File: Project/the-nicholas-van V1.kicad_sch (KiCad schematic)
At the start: 39 parts, among them J1 JST SH, J2 Pico EZmate, J3 USB_C sink board 1.3mm, J4 Conn_01x05, J5 ARGB, SW1 BOOT0, U1 STM32F401CBUx, U2 XC6206PxxxMR, U3 74AHCT1G125, Y1 8 MHz

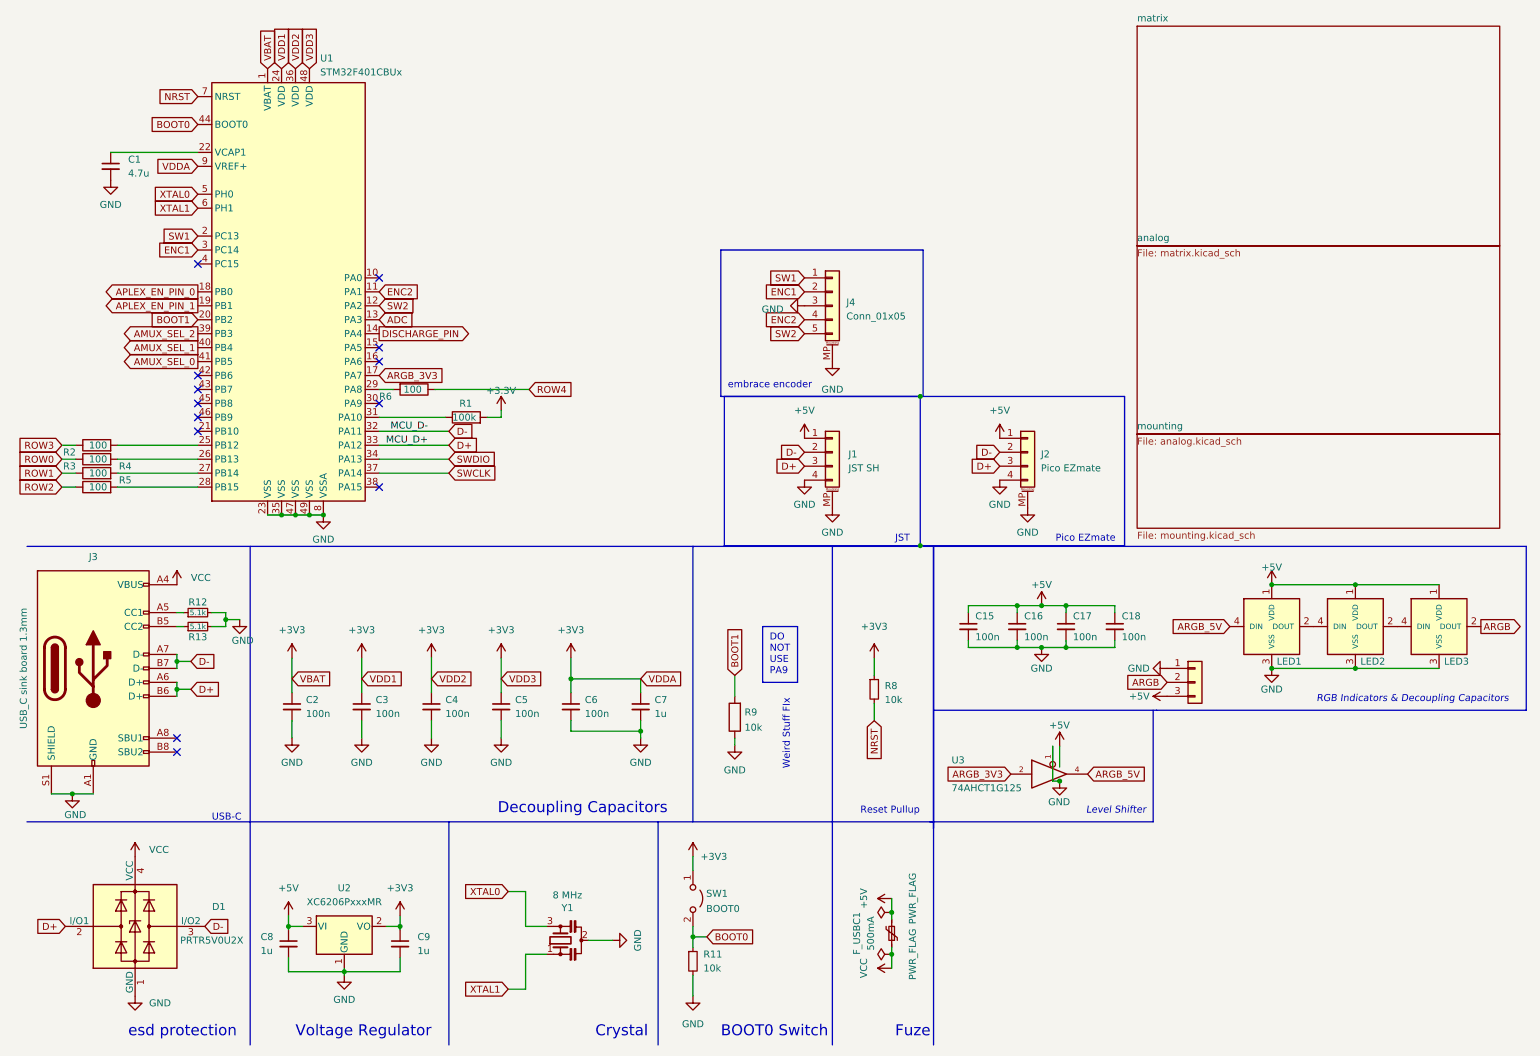
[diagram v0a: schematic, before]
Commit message: update revision
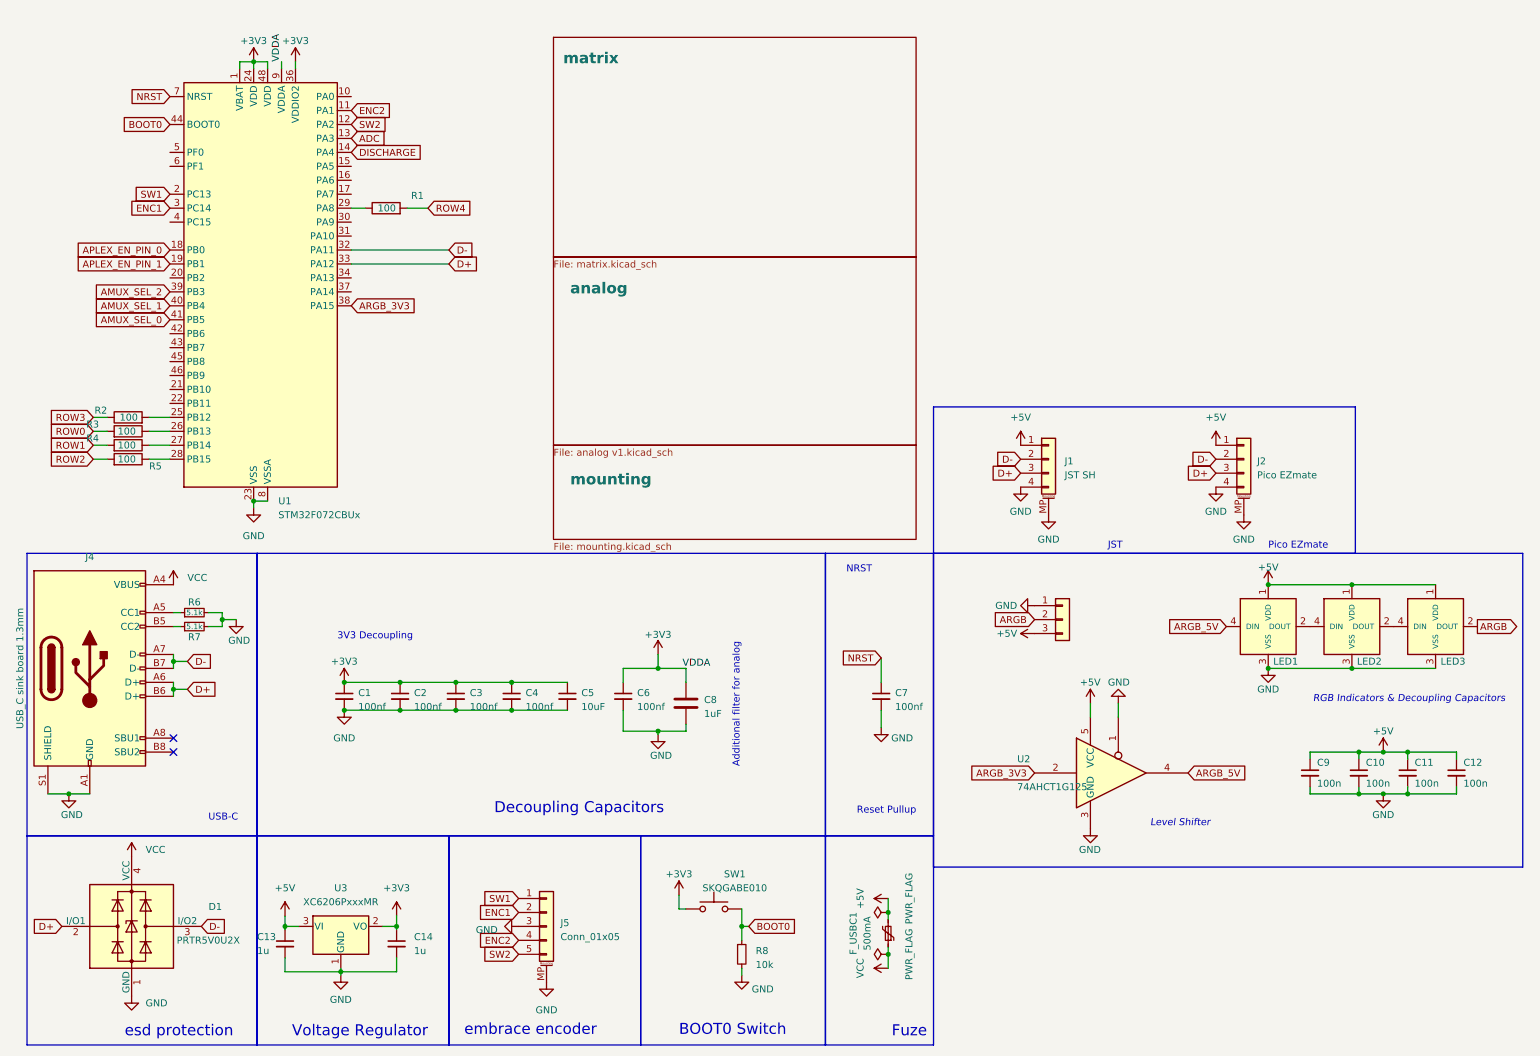
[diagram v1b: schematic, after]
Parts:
- removed R11: 10k, Resistor_SMD:R_0402_1005Metric, symbol Device:R_Small
- removed R6: 100, Resistor_SMD:R_0402_1005Metric, symbol Device:R
- removed R9: 10k, Resistor_SMD:R_0402_1005Metric, symbol Device:R
- removed SW1: BOOT0, Connector_PinHeader_2.54mm:PinHeader_1x02_P2.54mm_Vertical, symbol Jumper:Jumper_2_Open
- removed U1: STM32F401CBUx, Package_DFN_QFN:QFN-48-1EP_7x7mm_P0.5mm_EP5.6x5.6mm, symbol MCU_ST_STM32F4:STM32F401CBUx
- removed Y1: 8 MHz, Crystal:Resonator_SMD_Murata_CSTxExxV-3Pin_3.0x1.1mm, symbol Device:Resonator_Small
- added C8: 1uF, Capacitor_SMD:C_0402_1005Metric, symbol Device:C
- added SW1: SKQGABE010, Connector_PinSocket_2.54mm:PinSocket_1x02_P2.54mm_Vertical, symbol Switch:SW_Push
- added U1: STM32F072CBUx, Package_QFP:LQFP-48_7x7mm_P0.5mm, symbol MCU_ST_STM32F0:STM32F072CBUx
- C1: value 4.7u -> 100nf
- C2, C3, C4, C6: value 100n -> 100nf
- C5: value 100n -> 10uF
- C7: value 1u -> 100nf
- R1: value 100k -> 100; LCSC C25741 -> C25076
- renumbered C16 to C10, C17 to C11, C18 to C12, C8 to C13, C9 to C14, C15 to C9, J5 to J3, J3 to J4, J4 to J5, R12 to R6, R13 to R7, U3 to U2, U2 to U3
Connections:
- net +3V3: now also C1.1, C8.1, SW1.1, U1.1 (VBAT), U1.24 (VDD), U1.36 (VDDIO2), U1.48 (VDD), U1.9 (VDDA); no longer C7.1, R1.2, R8.1
- net ADC: now also U1.13 (PA3)
- net AMUX_SEL_0: now also U1.41 (PB5)
- net AMUX_SEL_1: now also U1.40 (PB4)
- net AMUX_SEL_2: now also U1.39 (PB3)
- net APLEX_EN_PIN_0: now also U1.18 (PB0)
- net APLEX_EN_PIN_1: now also U1.19 (PB1)
- net ARGB_3V3: now also U1.38 (PA15)
- net BOOT0: now also R8.1, SW1.2, U1.44 (BOOT0)
- net D+: now also U1.33 (PA12)
- net D-: now also U1.32 (PA11)
- net ENC1: now also U1.3 (PC14)
- net ENC2: now also U1.11 (PA1)
- net GND: now also R8.2, C8.2, U1.23 (VSS), U1.35 (VSS), U1.47 (VSS), U1.49 (VSS), U1.8 (VSSA)
- net NRST: now also C7.1, U1.7 (NRST); no longer R8.2
- net ROW0: now also R3.2; no longer R3.1
- net ROW1: now also R4.2; no longer R4.1
- net ROW2: now also R5.2; no longer R5.1
- net ROW4: now also R1.2
- net SW1: now also U1.2 (PC13)
- net SW2: now also U1.12 (PA2)
- net at R2.2: now also U1.25 (PB12)
- net at R1.1: now also U1.29 (PA8)
- new net: R3.1, U1.26 (PB13)
- new net: R5.1, U1.28 (PB15)
- new net: R4.1, U1.27 (PB14)
- new net DISCHARGE: U1.14 (PA4)
- no-connect marks 13 -> 2
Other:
- sheet analog: file analog.kicad_sch -> analog v1.kicad_sch
- note added: "3V3 Decoupling"
- note added: "Additional filter for analog"
- note added: "NRST"
- note removed: "Crystal"
- note removed: "DO NOT USE PA9"
- note removed: "Weird Stuff FIx"
- moved on the sheet: C10, C11, C12, C13, C14, C9, D1, F_USBC1, J1, J2, J4, J5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
